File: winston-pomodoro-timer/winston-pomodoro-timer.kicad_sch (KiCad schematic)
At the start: 42 parts, among them J1 Conn_01x05_Pin, J2 Conn_01x05_Pin, J4 Conn_01x04_Pin, J5 Conn_01x06_Pin, J6 UJC-HP-3-SMT-TR, U1 ATmega328P-A, U2 BQ24075RGT, Y1 Crystal_GND24

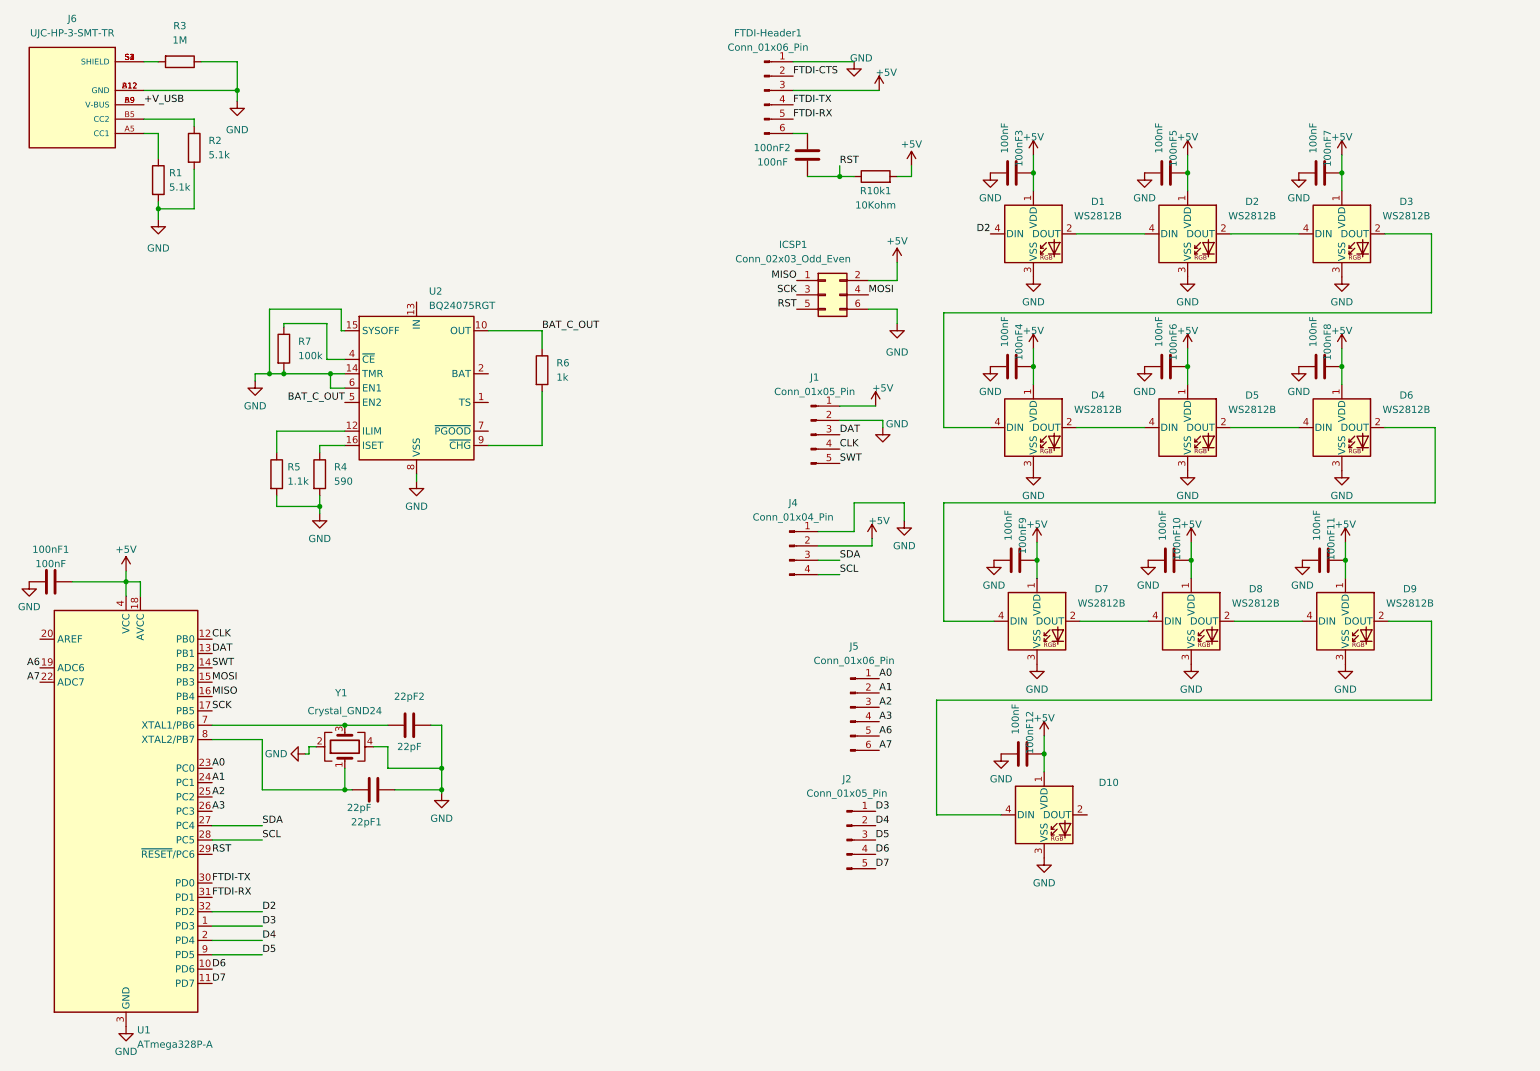
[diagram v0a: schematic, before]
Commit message: finished layout and routing
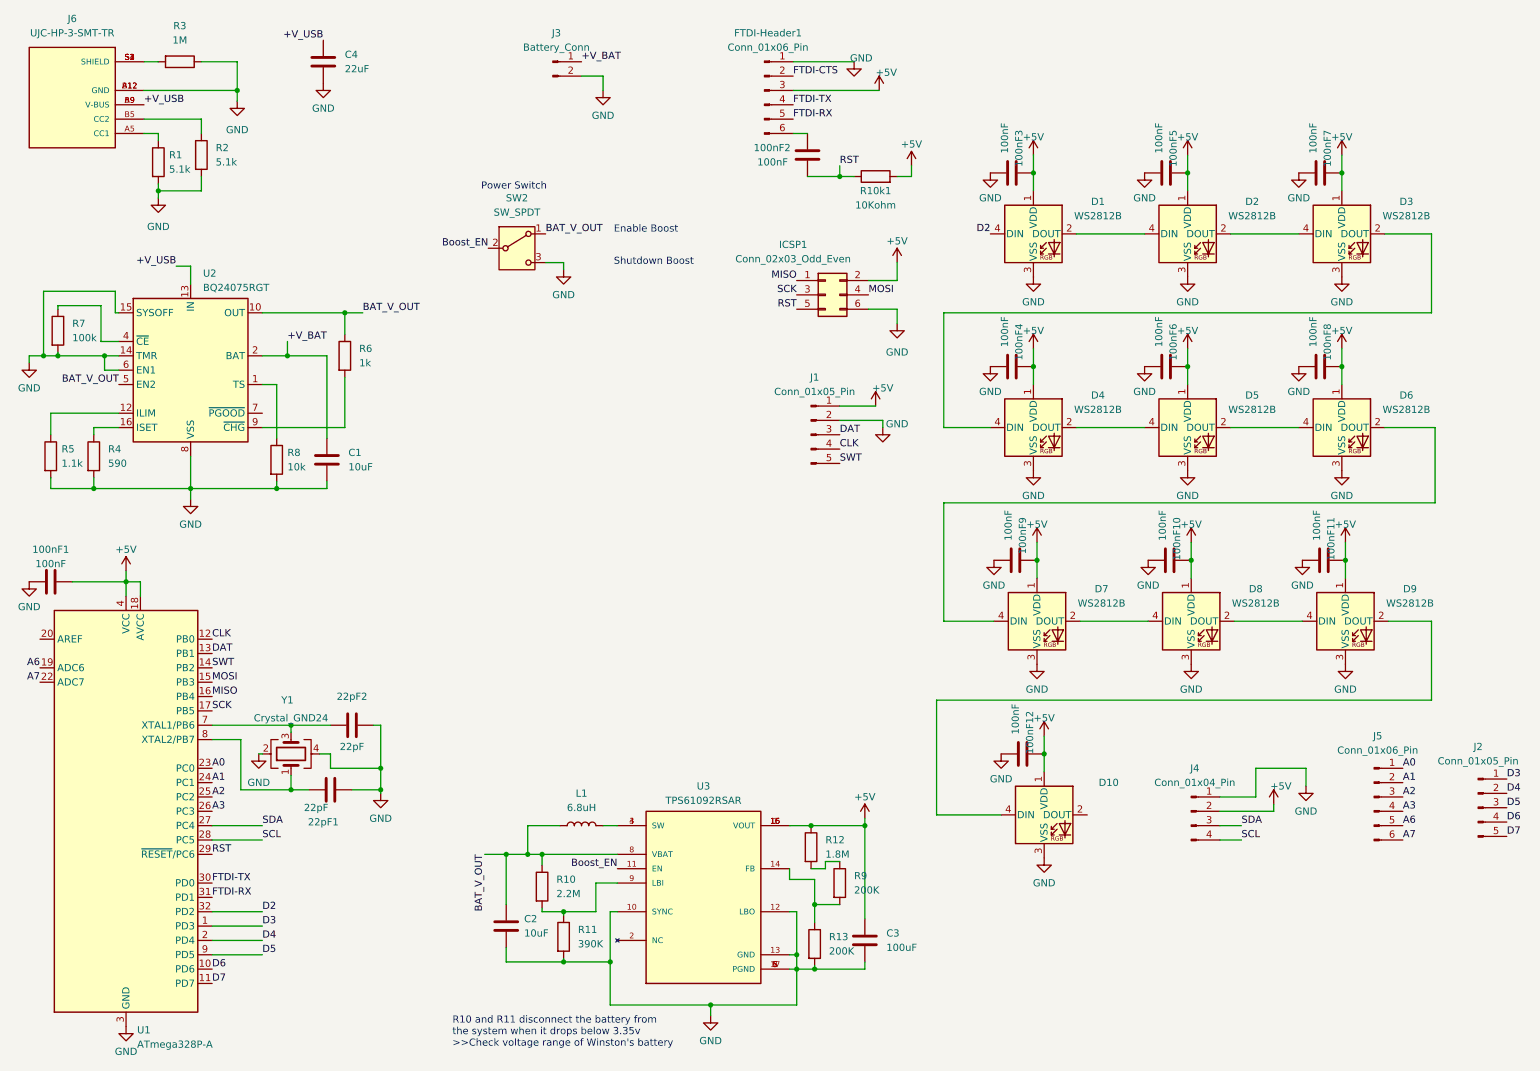
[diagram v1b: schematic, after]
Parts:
- added C1, C2: 10uF, Capacitor_SMD:C_0603_1608Metric, symbol Device:C
- added C3: 100uF, Capacitor_SMD:C_0805_2012Metric, symbol Device:C
- added C4: 22uF, Capacitor_SMD:C_0603_1608Metric, symbol Device:C
- added J3: Battery_Conn, Connector_PinSocket_2.00mm:PinSocket_1x02_P2.00mm_Vertical, symbol Connector:Conn_01x02_Pin
- added L1: 6.8uH, Inductor_SMD:L_Bourns-SRN4018, symbol Device:L
- added R10: 2.2M, Resistor_SMD:R_0603_1608Metric, symbol Device:R
- added R11: 390K, Resistor_SMD:R_0603_1608Metric, symbol Device:R
- added R12: 1.8M, Capacitor_SMD:C_0603_1608Metric, symbol Device:R
- added R13, R9: 200K, Resistor_SMD:R_0603_1608Metric, symbol Device:R
- added R8: 10k, Resistor_SMD:R_0603_1608Metric, symbol Device:R
- added SW2: SW_SPDT, Button_Switch_THT:SW_Slide_1P2T_CK_OS102011MS2Q, symbol Switch:SW_SPDT
- added U3: TPS61092RSAR, TPS61092RSAR:CONV_TPS61092RSAR, symbol TPS61092RSAR:TPS61092RSAR
- 100nF1, 100nF10, 100nF11, 100nF12, 100nF2, 100nF3, 100nF4, 100nF5, 100nF6, 100nF7, 100nF8, 100nF9, 22pF1, 22pF2: footprint Capacitor_SMD:C_0805_2012Metric_Pad1.18x1.45mm_HandSolder -> Capacitor_SMD:C_0603_1608Metric
- R1, R2, R3, R4, R5, R6, R7: footprint (none) -> Resistor_SMD:R_0603_1608Metric
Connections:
- net +5V: now also C3.1, R12.1, U3.1 (VOUT), U3.15 (VOUT), U3.16 (VOUT)
- net +V_USB: now also U2.13 (IN), C4.1
- net GND: now also C1.2, C2.2, C3.2, C4.2, J3.2 (Pin_2), R11.2, R13.2, R8.2, SW2.3 (C), U3.10 (SYNC), U3.12 (LBO), U3.13 (GND), U3.17 (PGND), U3.5 (PGND), U3.6 (PGND), U3.7 (PGND)
- net at U2.1 (TS): now also R8.1
- net +V_BAT: now reaches U2.2 (BAT), U2.3 (BAT)
- net +V_BAT: now also C1.1, J3.1 (Pin_1)
- net BAT_C_OUT renamed BAT_V_OUT
- net BAT_V_OUT: now also C2.1, L1.1, R10.1, SW2.1 (A), U3.8 (VBAT)
- new net: R10.2, R11.1, U3.9 (LBI)
- new net: R13.1, R9.2, U3.14 (FB)
- new net: L1.2, U3.3 (SW), U3.4 (SW)
- new net: R12.2, R9.1
- new net Boost_EN: SW2.2 (B), U3.11 (EN)
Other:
- note added: "Enable Boost"
- note added: "Power Switch"
- note added: "R10 and R11 disconnect the battery from the system when it drops below 3.35v >>Check voltage range of Winston's battery"
- note added: "Shutdown Boost"
- moved on the sheet: 22pF1, 22pF2, J2, J4, J5, R1, R2, R4, R5, R6, R7, U2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
